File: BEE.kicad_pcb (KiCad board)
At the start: 2 copper layers, 73 x 38 mm, 30 parts, among them J1 RPI1_header, J10 Conn_01x02, J11 Conn_01x02, J12 Conn_01x02, J2 BEE_header, J3 Conn_01x03, J4 Conn_01x06, J5 Conn_01x03, J6 Conn_01x05, J7 Conn_01x03, J8 Conn_01x08, J9 Conn_01x02, SW1 SW_Push, SW2 SW_Push, SW3 SW_Push, U1 MCP3008, U2 MCP4911

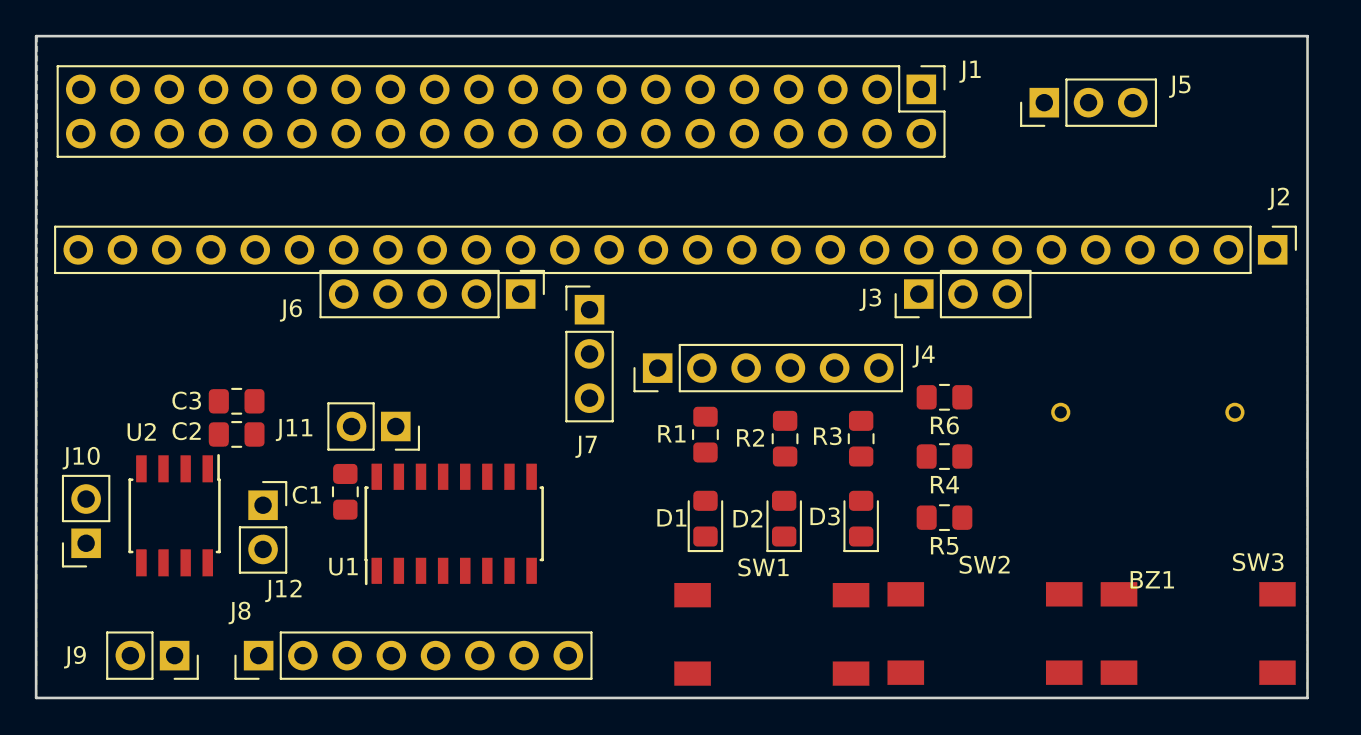
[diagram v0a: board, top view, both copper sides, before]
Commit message: wip: some traces added
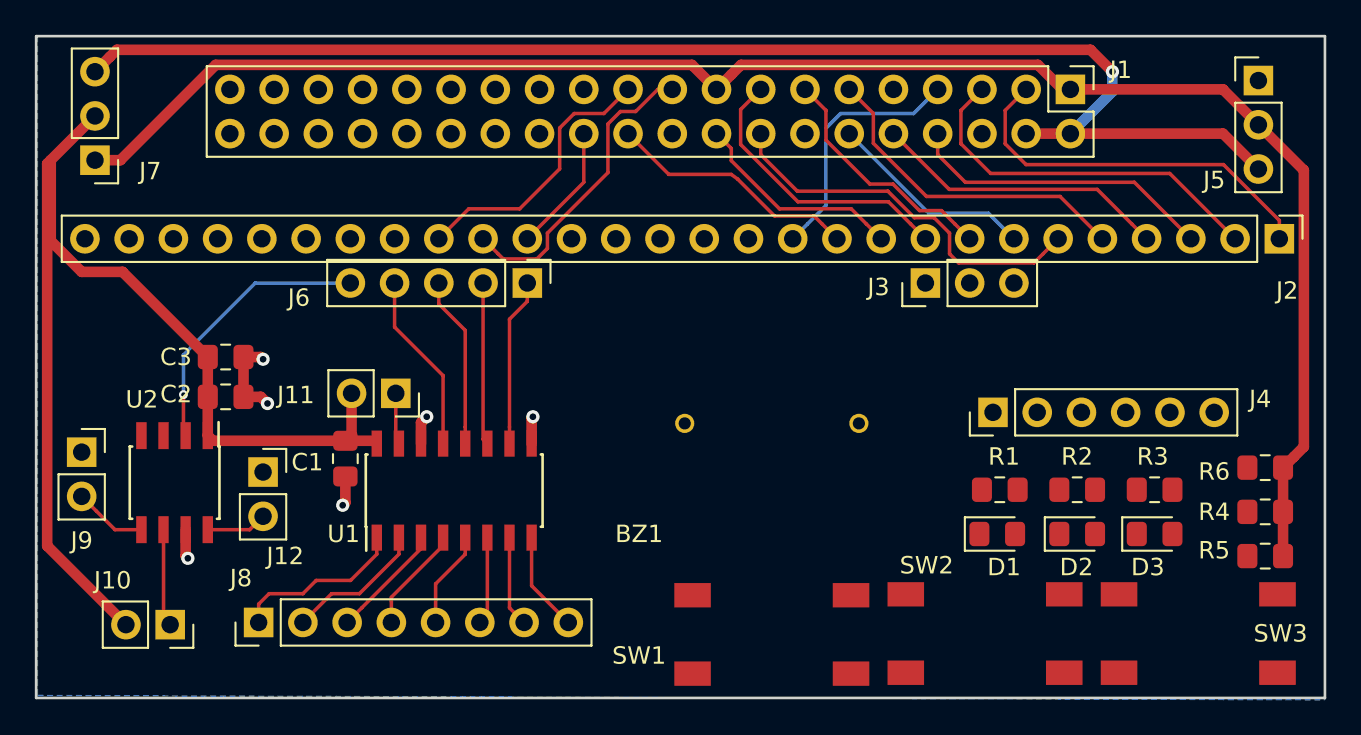
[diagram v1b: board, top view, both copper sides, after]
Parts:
- moved J7 29.7 mm to (103.4, 87.1), turned to 180 degrees
- moved BZ1 21.6 mm to (142.2, 102.2)
- moved J4 19.4 mm to (154.9, 101.6)
- moved R6 18.9 mm to (170.6, 104.8)
- moved R4 18.7 mm to (170.6, 107.3)
- moved R5 18.5 mm to (170.6, 109.9)
- moved R1 17.2 mm to (155.3, 106.0), turned to 0 degrees
- moved R3 17.1 mm to (164.2, 106.0), turned to 0 degrees
- moved R2 17.0 mm to (159.8, 106.0), turned to 0 degrees
- moved D3 16.9 mm to (164.2, 108.6), turned to 0 degrees
- moved D2 16.8 mm to (159.8, 108.6), turned to 0 degrees
- moved D1 16.8 mm to (155.2, 108.6), turned to 0 degrees
- moved J9 12.8 mm to (102.6, 103.9), turned to 0 degrees
- moved J5 12.4 mm to (170.2, 82.5), turned to 0 degrees
- moved J1 8.56 mm to (159.4, 83.1)
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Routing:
- net +3V3: track 0.00 -> 98.0 mm
- net +5V: track 0.00 -> 78.2 mm, vias 0 -> 1
- net VDD: track 0.00 -> 65.9 mm
- net /BCM2_SDA: track 0.00 -> 22.2 mm
- net /BCM23: track 0.00 -> 22.1 mm
- net /BCM3_SCL: track 0.00 -> 21.6 mm
- net /BCM17: track 0.00 -> 19.1 mm
- net /BCM14_TX: track 0.00 -> 17.7 mm
- net /BCM10_MOSI: track 0.00 -> 17.5 mm
- net /BCM15_RX: track 0.00 -> 17.0 mm
- net /BCM22_TRST: track 0.00 -> 16.5 mm
- net /CE_DAC: track 0.00 -> 16.0 mm, vias 0 -> 1
- net /BCM9_MISO: track 0.00 -> 15.8 mm
- net /BCM4_TDI: track 0.00 -> 14.5 mm
- net /BCM25_TCK: track 0.00 -> 14.5 mm
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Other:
- board size 73 x 38 mm -> 74 x 38 mm
- net class Default: clearance 0.2 -> 0.1524; trace_width 0.25 -> 0.1524; via_dia 0.8 -> 0.508; via_drill 0.4 -> 0.254
- net class Power: clearance 0.2 -> 0.254; trace_width 0.4572 -> 0.6096; via_dia 0.8 -> 0.762; via_drill 0.4 -> 0.381
- net class signal added: clearance 0.2032, trace_width 0.2032, via_dia 0.508, via_drill 0.254
- rule trace_clearance: 0.2 -> 0.1524
